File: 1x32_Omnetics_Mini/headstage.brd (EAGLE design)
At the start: 100 x 80 mm, 13 parts, among them U1 RHD2132_QFN

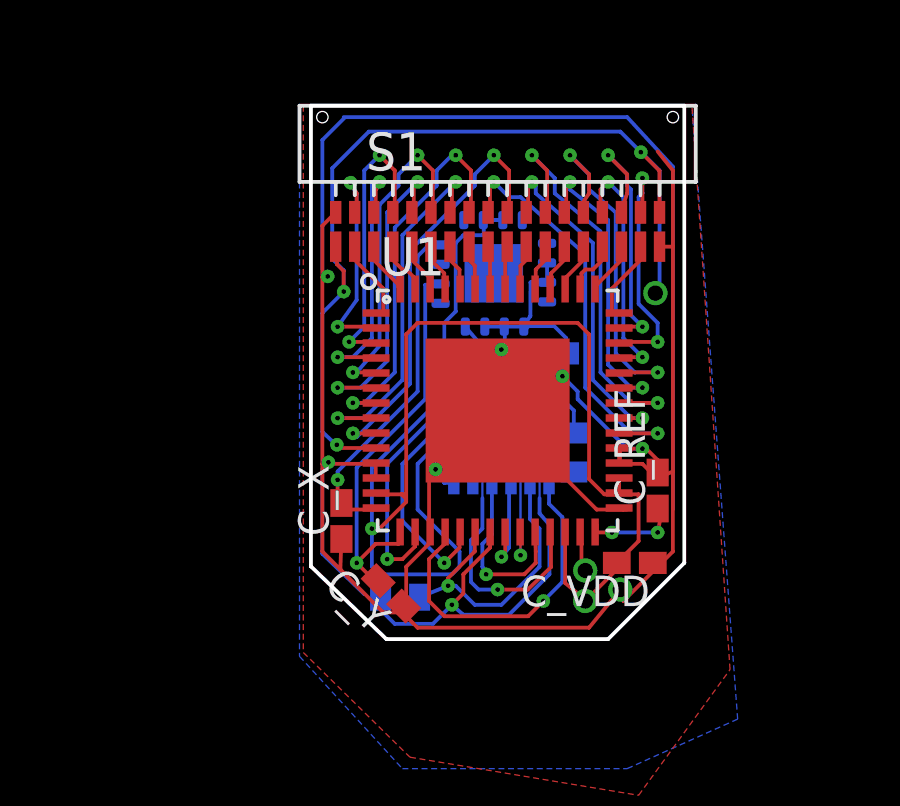
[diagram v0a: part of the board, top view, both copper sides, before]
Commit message: some cleanups
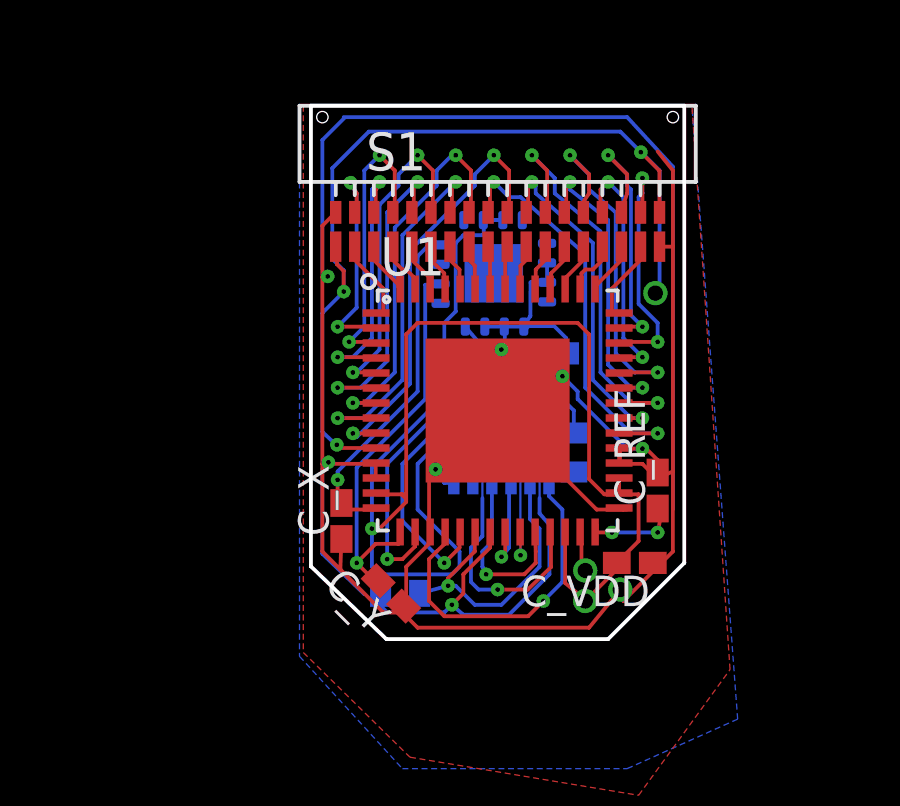
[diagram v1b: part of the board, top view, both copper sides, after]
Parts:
- moved R2 0.13 mm to (14.5, 13.0)
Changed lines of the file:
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@@
 <?xml version="1.0" encoding="utf-8"?>
 <!DOCTYPE eagle SYSTEM "eagle.dtd">
-<eagle version="7.5.0">
+<eagle version="6.3">
 <drawing>
 <settings>
@@
 <setting verticaltext="up"/>
 </settings>
-<grid distance="1" unitdist="mil" unit="mil" style="lines" multiple="1" display="yes" altdistance="0.025" altunitdist="inch" altunit="inch"/>
+<grid distance="5" unitdist="mil" unit="mil" style="lines" multiple="1" display="yes" altdistance="0.025" altunitdist="inch" altunit="inch"/>
 <layers>
 <layer number="1" name="Top" color="12" fill="1" visible="yes" active="yes"/>
@@
 <pass name="Default">
 <param name="RoutingGrid" value="50mil"/>
-<param name="AutoGrid" value="1"/>
-<param name="Efforts" value="0"/>
-<param name="TopRouterVariant" value="1"/>
 <param name="tpViaShape" value="round"/>
 <param name="PrefDir.1" value="|"/>
@@
 <element name="U1" library="RHD2000" package="QFN56_8_X_8_LARGE" value="RHD2132_QFN" x="17.78" y="19.05"/>
 <element name="R1" library="resistor" package="R0402" value="100" x="20.32" y="17.653" rot="MR90"/>
-<element name="R2" library="resistor" package="R0402" value="100" x="14.5288" y="12.827" rot="MR0"/>
+<element name="R2" library="resistor" package="R0402" value="100" x="14.5288" y="12.954" rot="MR0"/>
 <element name="R3" library="resistor" package="R0402" value="100" x="18.415" y="19.177" rot="MR180"/>
 <element name="C_A" library="resistor" package="C0402K" value="0.1uF" x="16.51" y="20.32" rot="MR270"/>
@@
 <contactref element="U1" pad="18"/>
 <wire x1="19.558" y1="16.5735" x2="19.4945" y2="16.637" width="0.127" layer="16"/>
-<wire x1="19.4945" y1="16.637" x2="19.4945" y2="15.9385" width="0.127" layer="16"/>
+<wire x1="19.4945" y1="16.637" x2="19.4945" y2="16.1925" width="0.127" layer="16"/>
 <wire x1="20.32" y1="17.003" x2="19.5095" y2="16.876" width="0.127" layer="16"/>
 <wire x1="19.5095" y1="16.876" x2="19.4945" y2="16.637" width="0.0762" layer="16"/>
-<wire x1="19.4945" y1="15.9385" x2="19.939" y2="15.494" width="0.127" layer="16"/>
-<wire x1="19.939" y1="15.494" x2="19.939" y2="13.335" width="0.127" layer="16"/>
+<wire x1="19.4945" y1="16.1925" x2="19.939" y2="15.748" width="0.127" layer="16"/>
+<wire x1="19.939" y1="15.748" x2="19.939" y2="13.335" width="0.127" layer="16"/>
 <wire x1="19.939" y1="13.335" x2="19.304" y2="12.7" width="0.127" layer="16"/>
 <via x="19.304" y="12.7" extent="1-16" drill="0.1524"/>
@@
 <wire x1="17.03" y1="15" x2="17.03" y2="14.871" width="0.127" layer="1"/>
 <wire x1="17.03" y1="14.871" x2="17.018" y2="14.859" width="0.127" layer="1"/>
-<wire x1="16.129" y1="13.208" x2="15.1788" y2="12.827" width="0.127" layer="16"/>
+<wire x1="16.129" y1="13.208" x2="15.1788" y2="12.954" width="0.127" layer="16"/>
 </signal>
 <signal name="SCLK+">
@@
 <contactref element="U1" pad="21"/>
 <contactref element="R2" pad="2"/>
-<wire x1="18.8595" y1="17.78" x2="19.05" y2="17.78" width="0.0762" layer="16"/>
-<wire x1="19.05" y1="17.78" x2="19.177" y2="17.653" width="0.0762" layer="16"/>
-<wire x1="19.177" y1="17.653" x2="19.177" y2="16.129" width="0.0762" layer="16"/>
+<wire x1="18.8595" y1="17.78" x2="19.05" y2="17.2466" width="0.0762" layer="16"/>
+<wire x1="19.05" y1="17.2466" x2="19.177" y2="17.1196" width="0.0762" layer="16"/>
+<wire x1="19.177" y1="17.1196" x2="19.177" y2="16.129" width="0.0762" layer="16"/>
 <wire x1="19.177" y1="16.129" x2="19.177" y2="15.621" width="0.127" layer="16"/>
 <wire x1="19.177" y1="15.621" x2="19.5072" y2="15.24" width="0.127" layer="16"/>
@@
 <wire x1="17.526" y1="14.605" x2="17.526" y2="14.996" width="0.0762" layer="1"/>
 <wire x1="17.526" y1="14.996" x2="17.53" y2="15" width="0.0762" layer="1"/>
-<wire x1="16.256" y1="12.573" x2="15.621" y2="11.938" width="0.127" layer="16"/>
-<wire x1="15.621" y1="11.938" x2="14.351" y2="11.938" width="0.127" layer="16"/>
-<wire x1="14.351" y1="11.938" x2="14.0058" y2="12.2832" width="0.127" layer="16"/>
-<wire x1="14.0058" y1="12.2832" x2="13.8788" y2="12.827" width="0.127" layer="16"/>
+<wire x1="16.256" y1="12.573" x2="16.002" y2="12.319" width="0.127" layer="16"/>
+<wire x1="16.002" y1="12.319" x2="14.097" y2="12.319" width="0.127" layer="16"/>
+<wire x1="14.097" y1="12.319" x2="13.8788" y2="12.5372" width="0.127" layer="16"/>
+<wire x1="13.8788" y1="12.5372" x2="13.8788" y2="12.954" width="0.127" layer="16"/>
 </signal>
 <signal name="MOSI+">
@@
 <contactref element="R3" pad="2"/>
 <wire x1="18.2245" y1="17.78" x2="18.161" y2="17.653" width="0.127" layer="16"/>
-<wire x1="18.161" y1="17.653" x2="18.415" y2="17.653" width="0.0762" layer="16"/>
-<wire x1="18.415" y1="17.653" x2="18.542" y2="17.526" width="0.0762" layer="16"/>
-<wire x1="18.542" y1="17.526" x2="18.542" y2="14.224" width="0.0762" layer="16"/>
+<wire x1="18.161" y1="17.653" x2="18.415" y2="17.2212" width="0.0762" layer="16"/>
+<wire x1="18.415" y1="17.2212" x2="18.542" y2="17.0942" width="0.0762" layer="16"/>
+<wire x1="18.542" y1="17.0942" x2="18.542" y2="14.224" width="0.0762" layer="16"/>
 <via x="18.542" y="14.224" extent="1-16" drill="0.1524"/>
 <wire x1="18.542" y1="14.224" x2="18.542" y2="14.859" width="0.0762" layer="1"/>
@@
 <wire x1="17.765" y1="19.177" x2="17.892" y2="19.065" width="0.0762" layer="16"/>
 <wire x1="17.892" y1="19.065" x2="17.907" y2="18.415" width="0.127" layer="16"/>
-<wire x1="17.907" y1="18.415" x2="17.907" y2="16.9545" width="0.0762" layer="16"/>
-<wire x1="17.907" y1="16.9545" x2="18.2245" y2="16.637" width="0.0762" layer="16"/>
+<wire x1="17.907" y1="18.415" x2="17.907" y2="17.145" width="0.0762" layer="16"/>
+<wire x1="17.907" y1="17.145" x2="18.2118" y2="16.8402" width="0.0762" layer="16"/>
+<wire x1="18.2118" y1="16.8402" x2="18.2245" y2="16.637" width="0.0762" layer="16"/>
 <wire x1="18.03" y1="15" x2="18.03" y2="14.9392" width="0.127" layer="1"/>
 <wire x1="18.03" y1="14.9392" x2="18.034" y2="14.9352" width="0.127" layer="1"/>
@@
 <contactref element="S2" pad="B4"/>
 <contactref element="U1" pad="24"/>
-<wire x1="17.5895" y1="16.637" x2="17.5895" y2="14.9225" width="0.127" layer="16"/>
-<wire x1="17.5895" y1="14.9225" x2="17.272" y2="14.605" width="0.127" layer="16"/>
-<wire x1="17.272" y1="14.605" x2="17.272" y2="13.843" width="0.127" layer="16"/>
+<wire x1="17.5895" y1="16.637" x2="17.5895" y2="14.6685" width="0.127" layer="16"/>
+<wire x1="17.5895" y1="14.6685" x2="17.272" y2="14.351" width="0.127" layer="16"/>
+<wire x1="17.272" y1="14.351" x2="17.272" y2="13.843" width="0.127" layer="16"/>
 <wire x1="17.272" y1="13.843" x2="17.399" y2="13.589" width="0.127" layer="16"/>
 <via x="17.399" y="13.589" extent="1-16" drill="0.1524"/>
@@
 <contactref element="U1" pad="25"/>
 <contactref element="S2" pad="T4"/>
-<wire x1="17.5895" y1="17.78" x2="17.526" y2="17.78" width="0.0762" layer="16"/>
-<wire x1="17.526" y1="17.78" x2="17.272" y2="17.653" width="0.0762" layer="16"/>
-<wire x1="17.272" y1="17.653" x2="17.272" y2="16.129" width="0.0762" layer="16"/>
-<wire x1="17.272" y1="16.129" x2="17.272" y2="15.113" width="0.127" layer="16"/>
-<wire x1="17.272" y1="15.113" x2="16.891" y2="14.732" width="0.127" layer="16"/>
-<wire x1="16.891" y1="14.732" x2="16.891" y2="13.335" width="0.127" layer="16"/>
+<wire x1="17.5895" y1="17.78" x2="17.526" y2="17.2974" width="0.0762" layer="16"/>
+<wire x1="17.526" y1="17.2974" x2="17.272" y2="17.1704" width="0.0762" layer="16"/>
+<wire x1="17.272" y1="17.1704" x2="17.272" y2="16.129" width="0.0762" layer="16"/>
+<wire x1="17.272" y1="16.129" x2="17.272" y2="14.859" width="0.127" layer="16"/>
+<wire x1="17.272" y1="14.859" x2="16.891" y2="14.478" width="0.127" layer="16"/>
+<wire x1="16.891" y1="14.478" x2="16.891" y2="13.335" width="0.127" layer="16"/>
 <wire x1="16.891" y1="13.335" x2="17.145" y2="13.081" width="0.127" layer="16"/>
 <wire x1="17.145" y1="13.081" x2="17.78" y2="13.081" width="0.127" layer="16"/>
@@
 <via x="12.446" y="21.844" extent="1-16" drill="0.1524"/>
 <wire x1="13.686" y1="21.844" x2="12.446" y2="21.844" width="0.127" layer="1"/>
-<wire x1="13.081" y1="26.289" x2="13.081" y2="22.733" width="0.127" layer="16"/>
-<wire x1="13.081" y1="22.733" x2="12.446" y2="21.844" width="0.127" layer="16"/>
+<wire x1="13.081" y1="26.289" x2="13.081" y2="22.479" width="0.127" layer="16"/>
+<wire x1="13.081" y1="22.479" x2="12.446" y2="21.844" width="0.127" layer="16"/>
 <contactref element="U1" pad="2"/>
 <contactref element="S1" pad="B2"/>
@@
 <wire x1="14.478" y1="26.924" x2="14.478" y2="26.543" width="0.127" layer="16"/>
 <wire x1="14.478" y1="26.543" x2="13.843" y2="25.908" width="0.127" layer="16"/>
-<wire x1="13.843" y1="25.908" x2="13.843" y2="21.209" width="0.127" layer="16"/>
+<wire x1="13.843" y1="25.908" x2="13.843" y2="21.082" width="0.127" layer="16"/>
 <via x="12.954" y="20.32" extent="1-16" drill="0.1524"/>
 <wire x1="12.954" y1="20.32" x2="13.081" y2="20.32" width="0.127" layer="16"/>
-<wire x1="13.081" y1="20.32" x2="13.843" y2="21.209" width="0.127" layer="16"/>
+<wire x1="13.081" y1="20.32" x2="13.843" y2="21.082" width="0.127" layer="16"/>
 <contactref element="U1" pad="5"/>
 <contactref element="S1" pad="B6"/>
@@
 <wire x1="13.843" y1="26.543" x2="13.843" y2="26.67" width="0.127" layer="1"/>
 <wire x1="12.446" y1="20.828" x2="12.954" y2="20.828" width="0.127" layer="16"/>
-<wire x1="13.843" y1="26.67" x2="13.589" y2="26.67" width="0.127" layer="16"/>
-<wire x1="13.589" y1="26.67" x2="13.589" y2="21.463" width="0.127" layer="16"/>
+<wire x1="13.843" y1="26.67" x2="13.589" y2="26.416" width="0.127" layer="16"/>
+<wire x1="13.589" y1="26.416" x2="13.589" y2="21.463" width="0.127" layer="16"/>
 <wire x1="13.589" y1="21.463" x2="12.954" y2="20.828" width="0.127" layer="16"/>
 <contactref element="U1" pad="4"/>
